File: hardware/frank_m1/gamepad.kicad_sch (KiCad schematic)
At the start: 4 parts, among them J5 Gamepad

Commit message: FRANK M1 HW Rev 1.00
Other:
- title: Frank M2 -> FRANK M1
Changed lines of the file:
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@@
 	(paper "A4")
 	(title_block
-		(title "Frank M2")
-		(date "2025-02-02")
-		(rev "1.01")
+		(title "FRANK M1")
+		(date "2025-02-04")
+		(rev "1.00")
 		(company "Mikhail Matveev")
 		(comment 1 "https://github.com/xtremespb/frank")

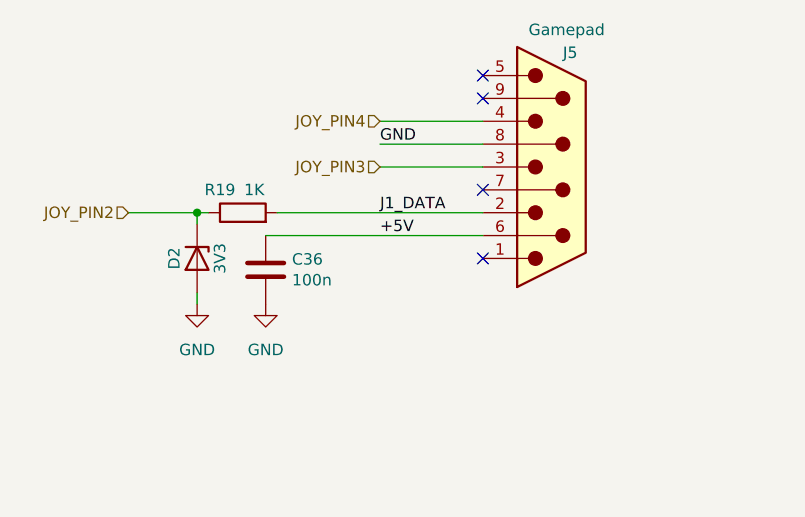
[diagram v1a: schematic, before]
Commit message: Names changed
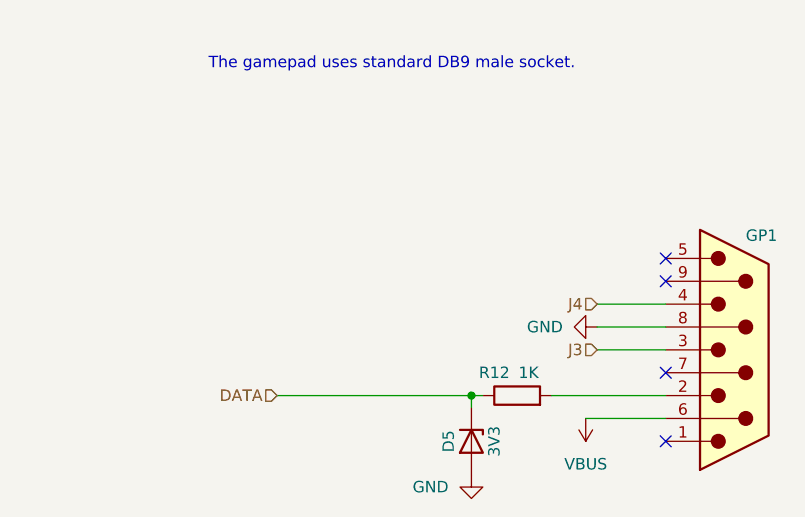
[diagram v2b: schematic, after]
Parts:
- removed C36: 100n, FRANK:Capacitor (0805), symbol Device:C
- removed D2: 3V3, FRANK:Diode (SOD-323), symbol Device:D_Zener
- removed J5: Gamepad, FRANK:D-SUB (9 pin, male, top mount), symbol FRANK:DB9_Male_Small
- removed R19: 1K, FRANK:Resistor (0805), symbol Device:R
- added D5: 3V3, FRANK:Diode (SOD-323), symbol Device:D_Zener
- added GP1: D-SUB 9 Male, FRANK:D-SUB (9 pin, male, top mount), symbol FRANK:DB9_Male_Small
- added R12: 1K, FRANK:Resistor (0805), symbol Device:R
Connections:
- net GND: now also D5.2 (A), GP1.8
- new net: GP1.2, R12.2
- new net DATA: D5.1 (K), R12.1
- new net J3: GP1.3
- new net J4: GP1.4
- new net VBUS: GP1.6
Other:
- note added: "The gamepad uses standard DB9 male socket."
- title: FRANK M1 -> FRANK

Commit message: FRANK M1 & M2 HW Revisions
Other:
- title: FRANK -> FRANK M1
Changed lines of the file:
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@@
 	(paper "A4")
 	(title_block
-		(title "FRANK")
+		(title "FRANK M1")
 		(date "2025-02-18")
 		(rev "1.13")
